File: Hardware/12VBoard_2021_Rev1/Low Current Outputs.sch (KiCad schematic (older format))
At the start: 54 parts

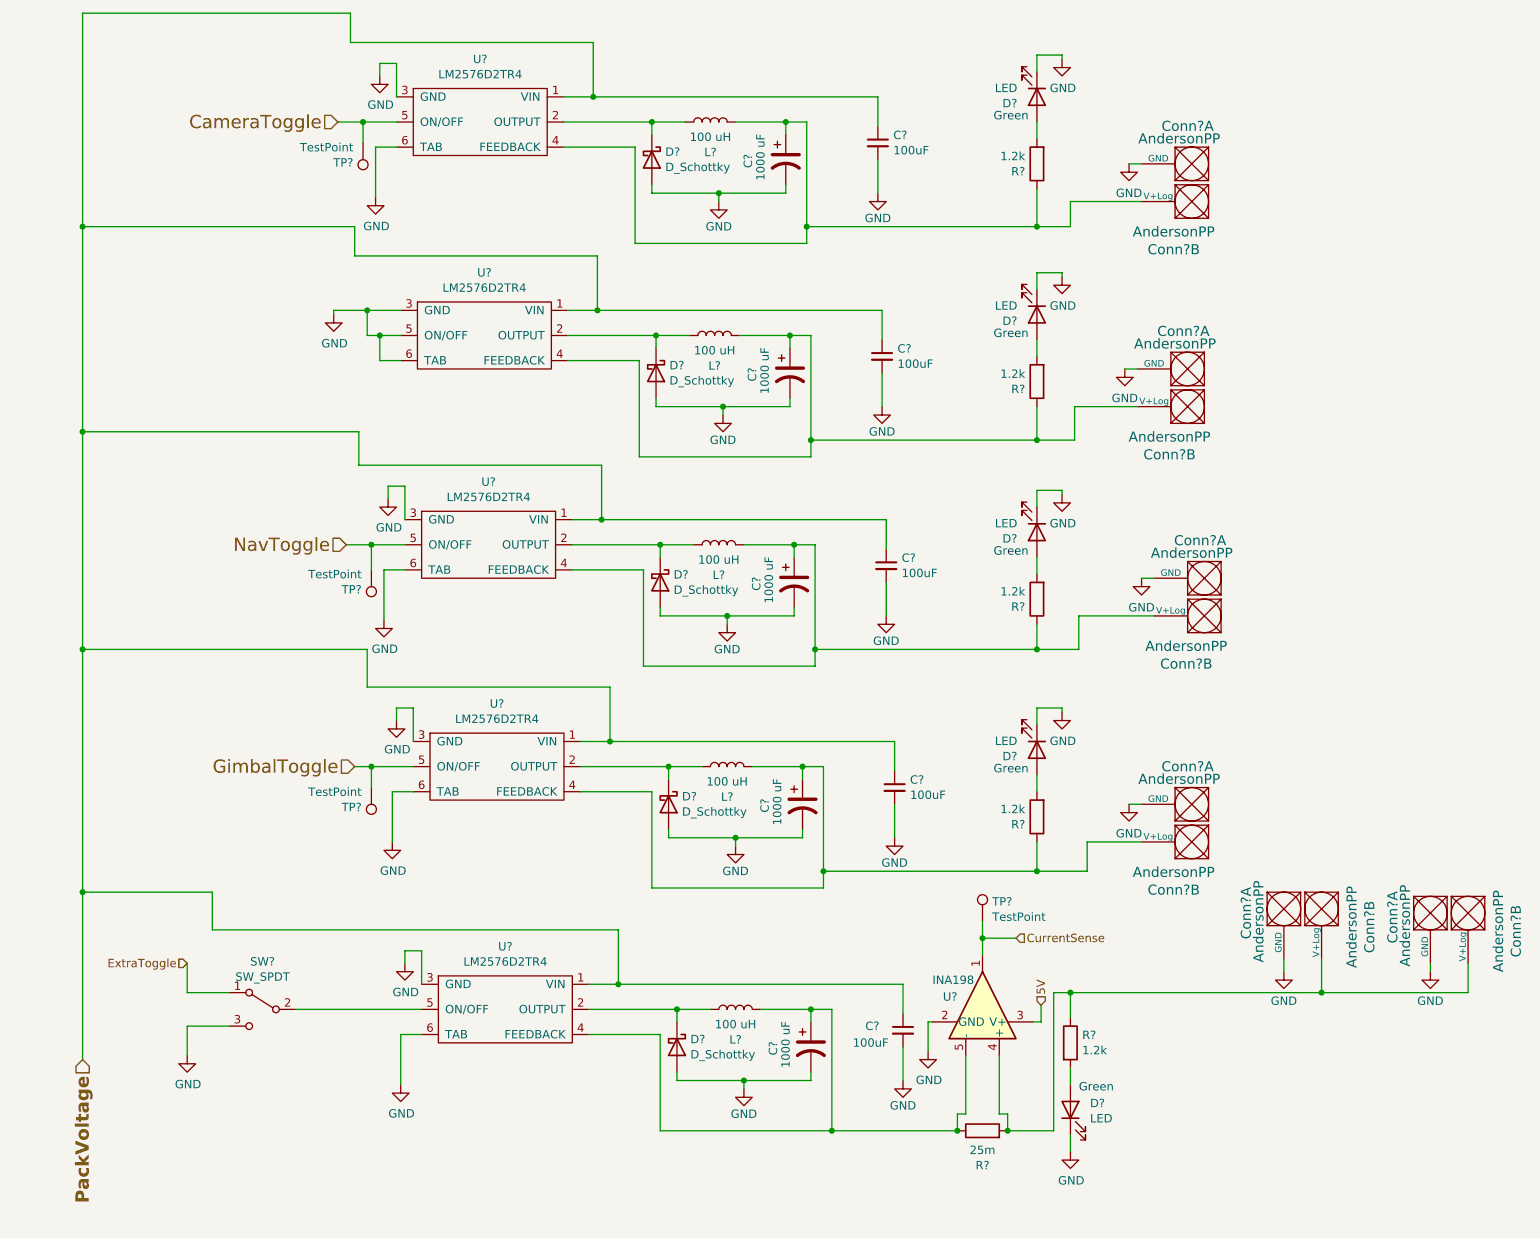
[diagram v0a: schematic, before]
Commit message: Changed things
Dans a quitter
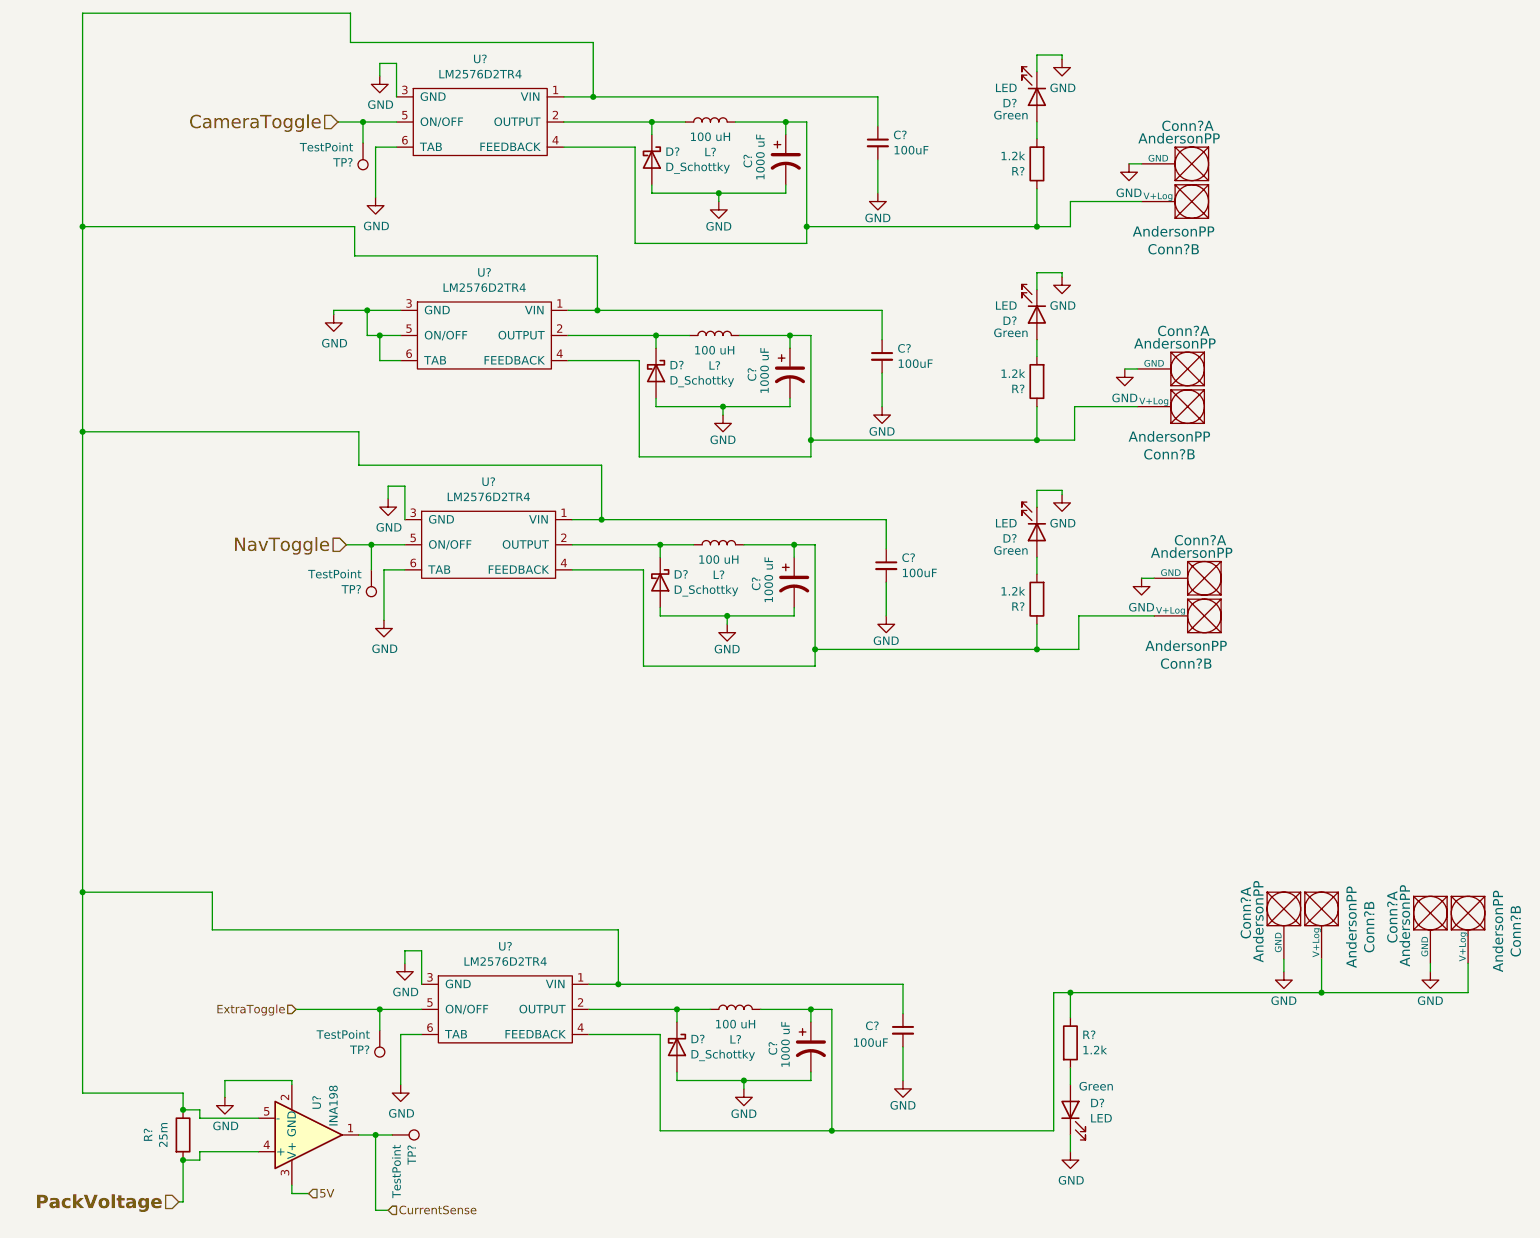
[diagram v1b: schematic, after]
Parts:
- removed C?: 1000 uF, symbol Device:CP1
- removed C?: 100uF, symbol Device:C_Small
- removed Conn? (x2): AndersonPP, symbol MRDT_Connectors:AndersonPP
- removed D?: D_Schottky, symbol Device:D_Schottky
- removed D?: LED, symbol Device:LED
- removed L?: 100 uH, Inductor_SMD:L_0603_1608Metric_Pad1.05x0.95mm_HandSolder, symbol Device:L
- removed R?: 25m, symbol Device:R
- removed R?: 1.2k, symbol Device:R
- removed SW?: SW_SPDT, symbol Switch:SW_SPDT
- removed TP? (x2): TestPoint, symbol Connector:TestPoint
- removed U?: LM2576D2TR4, MRDT_Devices:LM2576, symbol 12VBoard_2021_Rev1-rescue:LM2576D2TR4-MRDT_Devices
- removed U?: INA198, Package_TO_SOT_SMD:SOT-23-5, symbol Amplifier_Current:INA198
- added R?: 25m, symbol Device:R
- added TP? (x2): TestPoint, symbol Connector:TestPoint
- added U?: INA198, Package_TO_SOT_SMD:SOT-23-5, symbol Amplifier_Current:INA198
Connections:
- net 5V: now also U?.3 (V+)
- net CurrentSense: now also TP?.1, U?.1
- net ExtraToggle: now also U?.5 (ON/OFF), TP?.1
- net GND: now also U?.2 (GND)
- net PackVoltage: now also R?.2, U?.4 (+); no longer C?.1, C?.1, C?.1, C?.1, U?.1 (VIN), U?.1 (VIN), U?.1 (VIN), U?.1 (VIN)
- net at C?.1, L?.2, U?.4 (FEEDBACK): now also Conn?.2 (V+Log), Conn?.2 (V+Log), R?.1
- new net: C?.1, C?.1, C?.1, C?.1, R?.1, U?.1 (VIN), U?.1 (VIN), U?.1 (VIN), U?.1 (VIN), U?.5 (-)
